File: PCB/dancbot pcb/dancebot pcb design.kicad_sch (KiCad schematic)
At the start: 26 parts, among them J1 ESP32-PICO-KIT-V4.1, J2 Voltage Regulator, J4 Pins, J6 Conn_01x04_Socket, J7 Conn_01x04_Socket, Q2 PMOS, Q3 2N3904, Q4 PMOS, Q5 PMOS, SW1 SP switch, SW2 SW_SPST

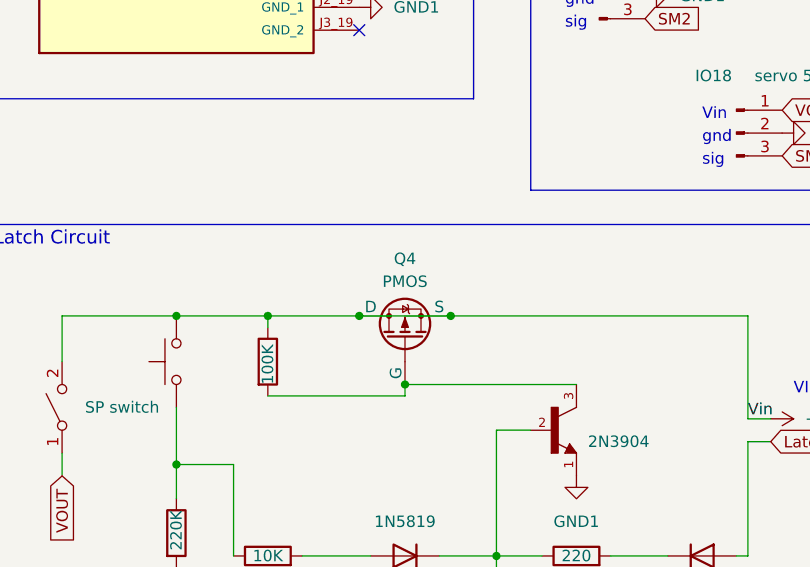
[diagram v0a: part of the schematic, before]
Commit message: Connections For Layout Revision 2
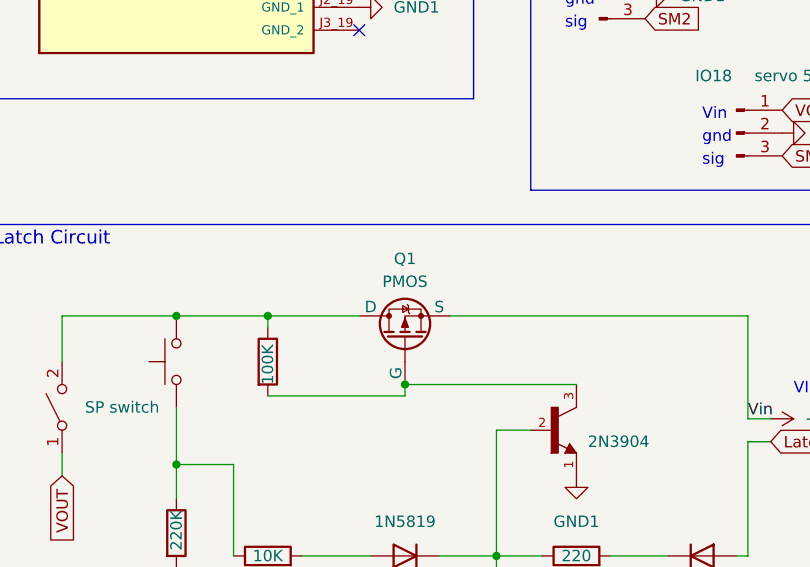
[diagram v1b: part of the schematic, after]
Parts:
- removed Q4: PMOS, dancebot pcb libraries stuff:TO254P1052X465X1989-3, symbol Simulation_SPICE:PMOS
- added Q1: PMOS, dancebot pcb libraries stuff:TO254P1052X465X1989-3, symbol Simulation_SPICE:PMOS
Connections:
- net +5V: now also Q1.3 (S); no longer R5.1, SW1.2, SW2.2 (B)
- net at Q3.3, R5.2: now also Q1.2 (G)
- new net: Q1.1 (D), R5.1, SW1.2, SW2.2 (B)
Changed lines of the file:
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@@
 (kicad_sch (version 20230121) (generator eeschema)
   (paper "A4")
-  (junction (at 72.39 137.16) (diameter 0) (color 0 0 0 0)
-  )
   (junction (at 111.76 50.8) (diameter 0) (color 0 0 0 0)
   )
@@
   )
   (junction (at 77.47 163.83) (diameter 0) (color 0 0 0 0)
-  )
-  (junction (at 62.23 137.16) (diameter 0) (color 0 0 0 0)
   )
   (junction (at 121.92 48.26) (diameter 0) (color 0 0 0 0)
@@
     (stroke (width 0) (type default))
   )
-  (wire (pts (xy 62.23 137.16) (xy 72.39 137.16))
-    (stroke (width 0) (type default))
-  )
   (wire (pts (xy 41.91 153.67) (xy 48.26 153.67))
     (stroke (width 0) (type default))
@@
         (path "/a5572283-9a9d-4246-8741-667ff8a68ceb"
           (reference "R5") (unit 1)
+        )
+      )
+    )
+  )
+  (symbol (lib_id "Simulation_SPICE:PMOS") (at 67.31 139.7 90) (unit 1)
+    (in_bom yes) (on_board yes) (dnp no) (fields_autoplaced)
+    (property "Reference" "Q1" (at 67.31 130.81 90)
+      (effects (font (size 1.27 1.27)))
+    )
+    (property "Value" "PMOS" (at 67.31 133.35 90)
+      (effects (font (size 1.27 1.27)))
+    )
+    (property "Footprint" "dancebot pcb libraries stuff:TO254P1052X465X1989-3" (at 64.77 134.62 0)
+      (effects (font (size 1.27 1.27)) hide)
+    )
+    (property "Datasheet" "https://ngspice.sourceforge.io/docs/ngspice-manual.pdf" (at 80.01 139.7 0)
+      (effects (font (size 1.27 1.27)) hide)
+    )
+    (property "Sim.Device" "PMOS" (at 84.455 139.7 0)
+      (effects (font (size 1.27 1.27)) hide)
+    )
+    (property "Sim.Type" "VDMOS" (at 86.36 139.7 0)
+      (effects (font (size 1.27 1.27)) hide)
+    )
+    (property "Sim.Pins" "1=D 2=G 3=S" (at 82.55 139.7 0)
+      (effects (font (size 1.27 1.27)) hide)
+    )
+    (pin "1")
+    (pin "2")
+    (pin "3")
+    (instances
+      (project "dancebot pcb design"
+        (path "/a5572283-9a9d-4246-8741-667ff8a68ceb"
+          (reference "Q1") (unit 1)
         )
       )
@@
         )
       )
-    )
-  )
-  (symbol (lib_id "Simulation_SPICE:PMOS") (at 67.31 139.7 90) (unit 1)
-    (in_bom yes) (on_board yes) (dnp no) (fields_autoplaced)
-    (property "Reference" "Q4" (at 67.31 130.81 90)
-      (effects (font (size 1.27 1.27)))
-    )
-    (property "Value" "PMOS" (at 67.31 133.35 90)
-      (effects (font (size 1.27 1.27)))
-    )
-    (property "Footprint" "dancebot pcb libraries stuff:TO254P1052X465X1989-3" (at 64.77 134.62 0)
-      (effects (font (size 1.27 1.27)) hide)
-    )
-    (property "Datasheet" "https://ngspice.sourceforge.io/docs/ngspice-manual.pdf" (at 80.01 139.7 0)
-      (effects (font (size 1.27 1.27)) hide)
-    )
-    (property "Sim.Device" "PMOS" (at 84.455 139.7 0)
-      (effects (font (size 1.27 1.27)) hide)
-    )
-    (property "Sim.Type" "VDMOS" (at 86.36 139.7 0)
-      (effects (font (size 1.27 1.27)) hide)
-    )
-    (property "Sim.Pins" "1=D 2=G 3=S" (at 82.55 139.7 0)
-      (effects (font (size 1.27 1.27)) hide)
-    )
-    (pin "1")
-    (pin "2")
-    (pin "3")
-    (instances
-      (project "dancebot pcb design"
-        (path "/a5572283-9a9d-4246-8741-667ff8a68ceb"
-          (reference "Q4") (unit 1)
-        )
-      )
